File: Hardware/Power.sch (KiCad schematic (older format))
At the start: 38 parts, among them J6 Barrel_Jack_MountingPin, U10 LM2734Y, U8 LM2734Y, U9 TPS63700DRCT

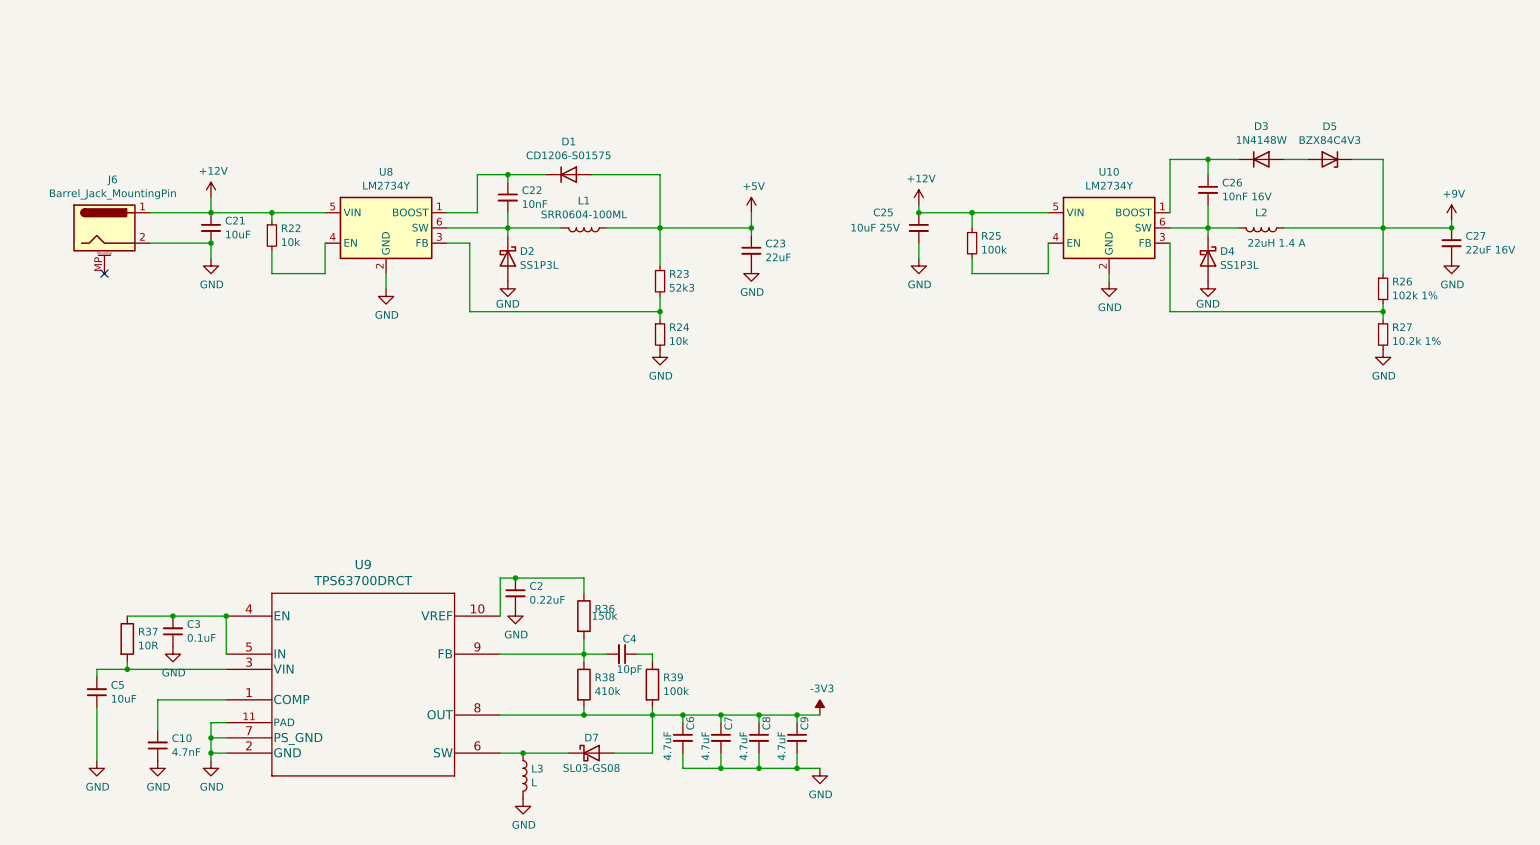
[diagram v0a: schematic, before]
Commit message: fixed -3V supply
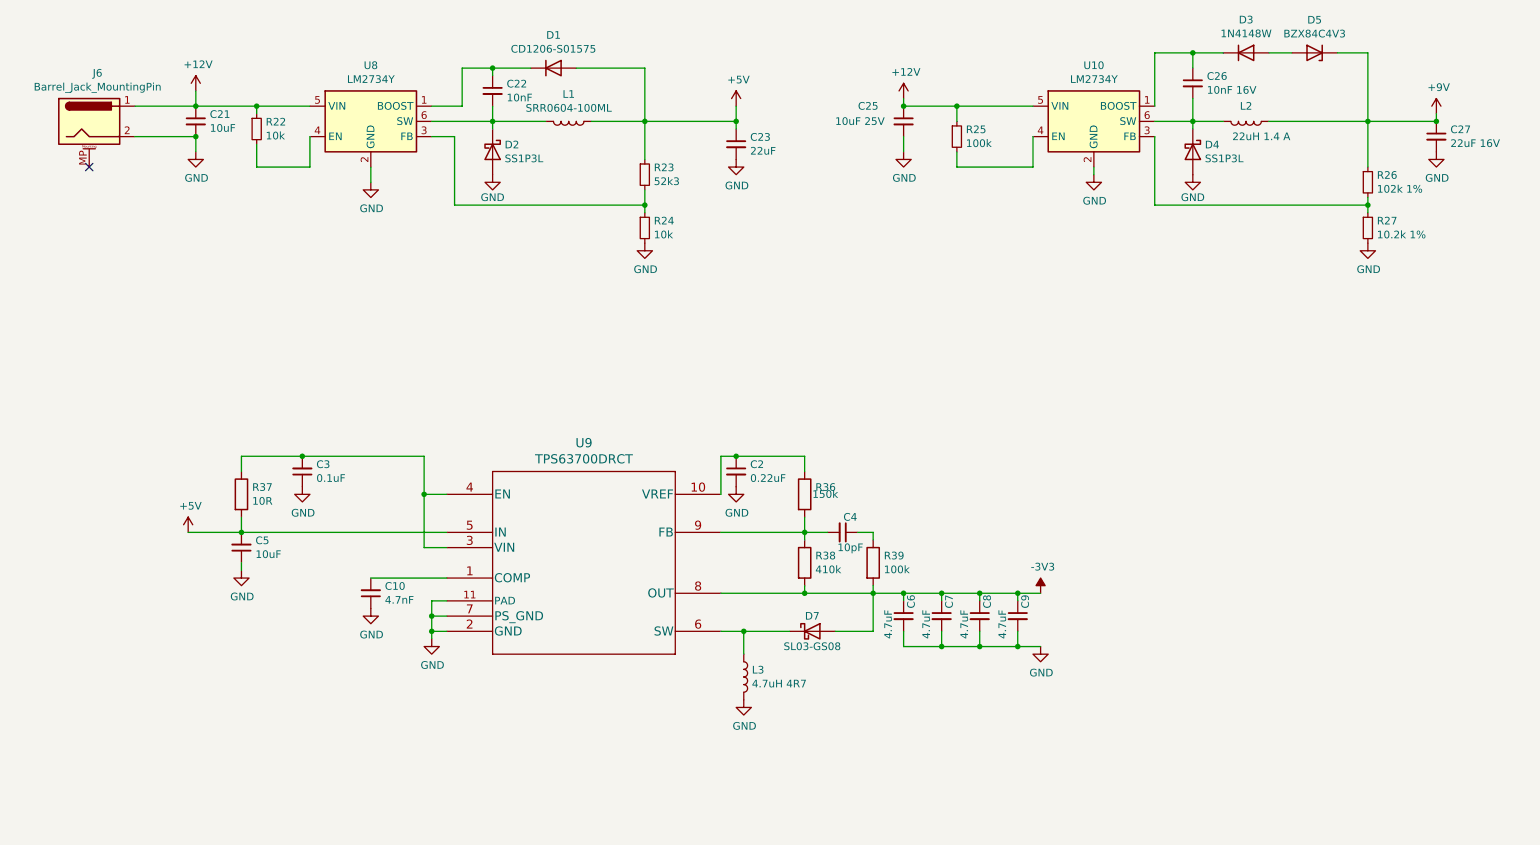
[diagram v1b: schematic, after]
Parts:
- L3: value L -> 4.7uH 4R7
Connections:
- net +5V: now also C5.2, R37.2, U9.5 (IN)
- net at C3.2, R37.1, U9.4 (EN): now also U9.3 (VIN); no longer U9.5 (IN)
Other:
- moved on the sheet: C10, C2, C21, C22, C23, C25, C26, C27, C3, C4, C5, C6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
